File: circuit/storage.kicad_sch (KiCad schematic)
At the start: 23 parts, among them J1 Port B, J15 TX (debug), J16 ISCP header, J2 Port C, J3 SDCard, J4 Port A, J43 Port G, U11 ATtiny2313-20P, U19 4013, U8 74HC595, Y1 16Mhz

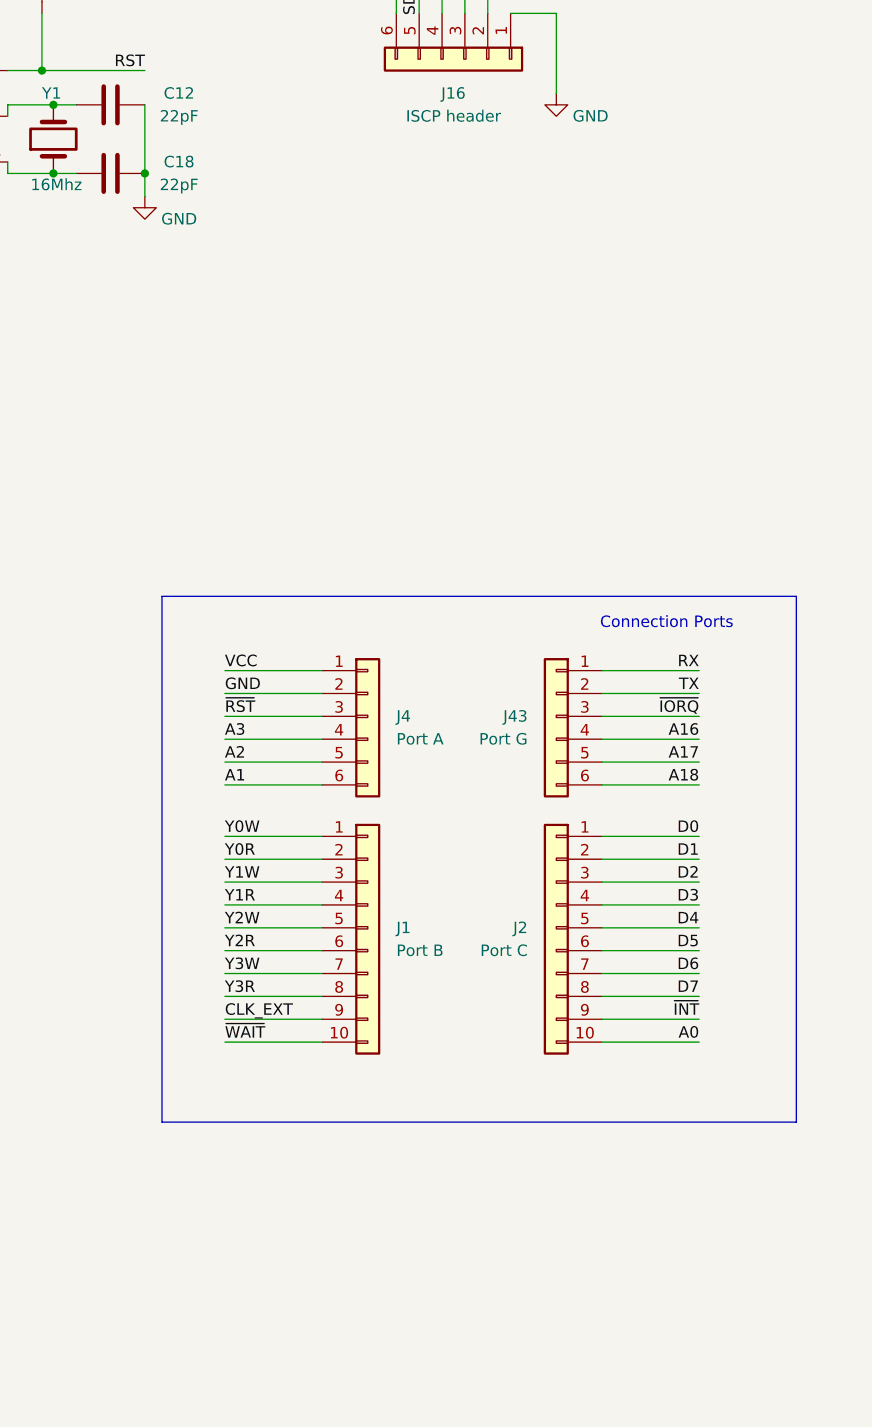
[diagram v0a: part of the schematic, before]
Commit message: Redeployt
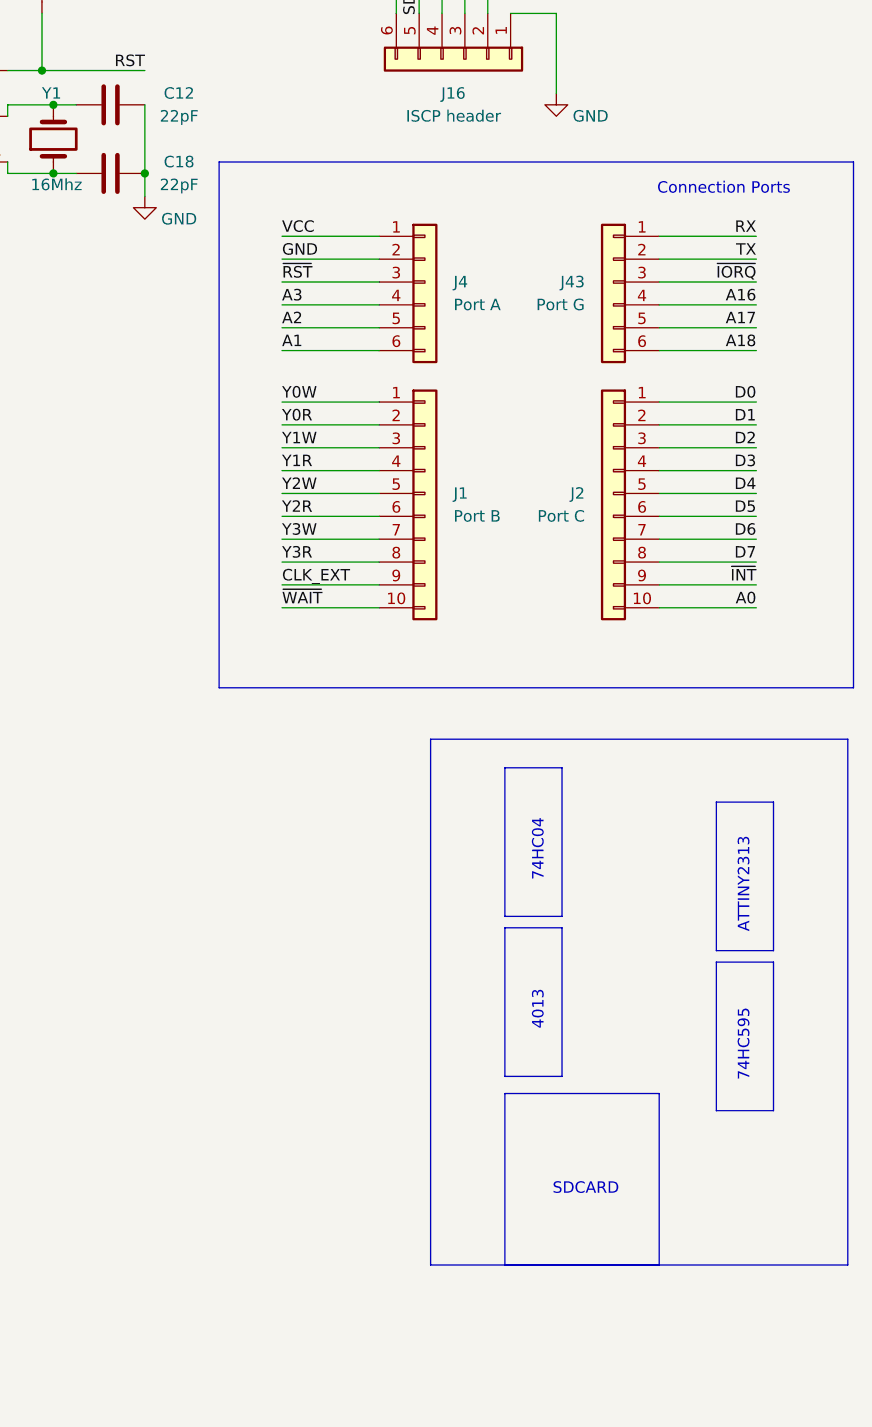
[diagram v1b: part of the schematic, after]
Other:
- note added: "4013"
- note added: "74HC04"
- note added: "74HC595"
- note added: "ATTINY2313"
- moved on the sheet: J1, J2, J4, J43
